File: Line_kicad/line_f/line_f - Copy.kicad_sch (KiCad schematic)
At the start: 15 parts, among them M2 Motor_DC, M3 Motor_DC, SW1 SW_SPST, SW2 SW_SPDT, SW3 SW_Push, SW4 SW_Push, U1 TB6612FNG_LINE, m1 BLACKPILL

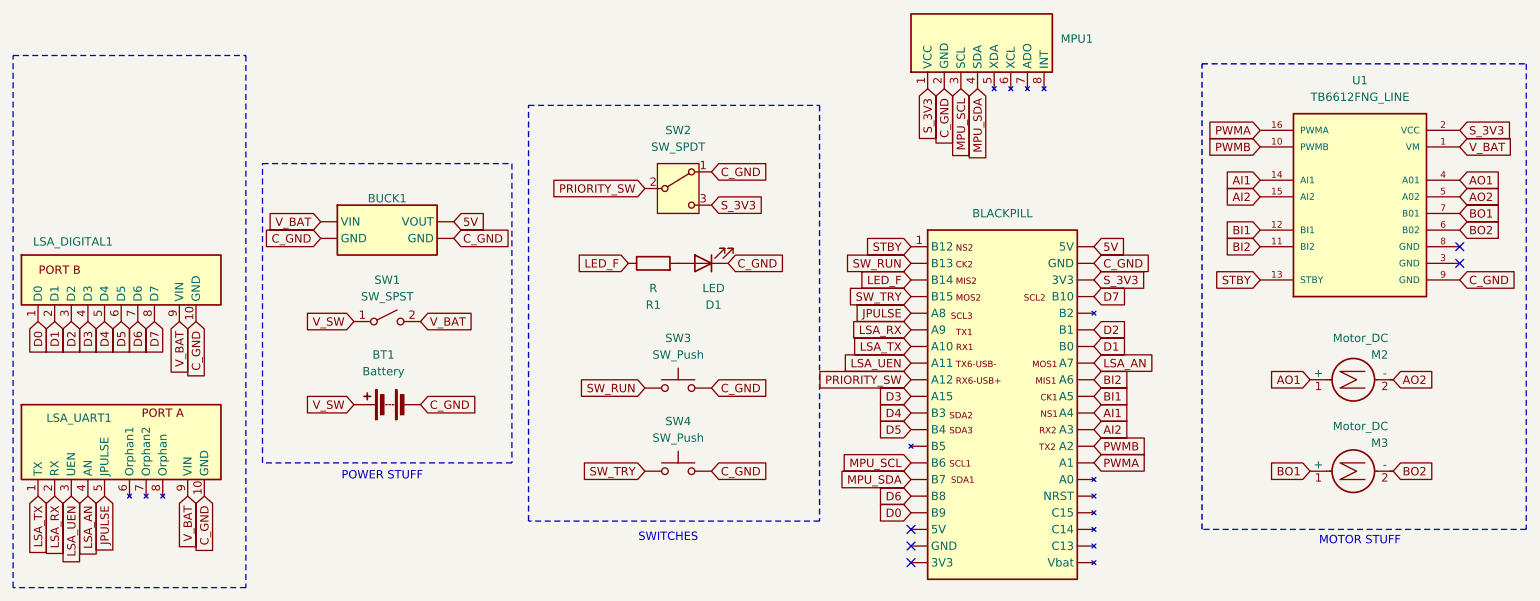
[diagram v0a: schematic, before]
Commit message: 3#
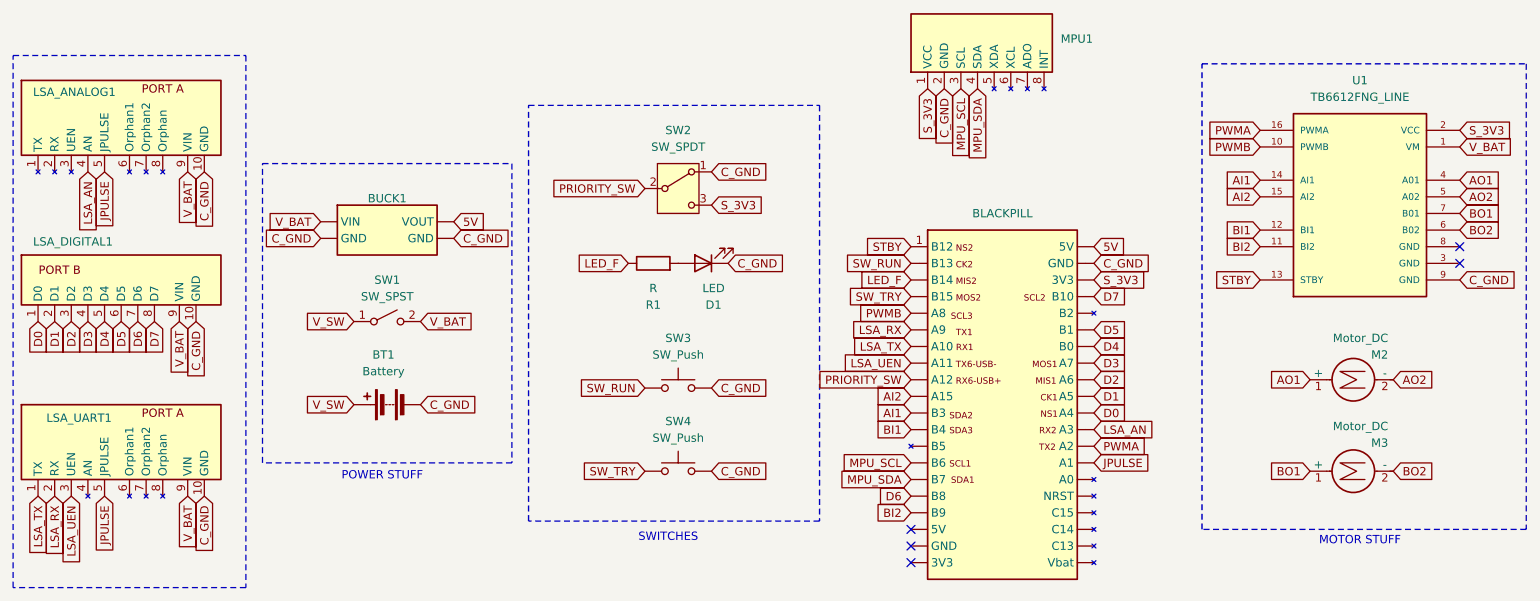
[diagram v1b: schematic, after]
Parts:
- added LSA_ANALOG1: ~, LINE_F_FOOT_LIB:LSA_ANALOG, symbol LINE_F_SYM_LIB:LSA_ANALOG
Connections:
- net AI1: now also m1.11 (B3); no longer m1.31 (A4)
- net AI2: now also m1.10 (A15); no longer m1.32 (A3)
- net BI1: now also m1.12 (B4); no longer m1.30 (A5)
- net BI2: now also m1.17 (B9); no longer m1.29 (A6)
- net C_GND: now also LSA_ANALOG1.10 (GND)
- net D0: now also m1.31 (A4); no longer m1.17 (B9)
- net D1: now also m1.30 (A5); no longer m1.27 (B0)
- net D2: now also m1.29 (A6); no longer m1.26 (B1)
- net D3: now also m1.28 (A7); no longer m1.10 (A15)
- net D4: now also m1.27 (B0); no longer m1.11 (B3)
- net D5: now also m1.26 (B1); no longer m1.12 (B4)
- net JPULSE: now also m1.34 (A1), LSA_ANALOG1.5 (JPULSE); no longer m1.5 (A8)
- net LSA_AN: now also m1.32 (A3), LSA_ANALOG1.4 (AN); no longer LSA_UART1.4 (AN), m1.28 (A7)
- net PWMA: now also m1.33 (A2); no longer m1.34 (A1)
- net PWMB: now also m1.5 (A8); no longer m1.33 (A2)
- net V_BAT: now also LSA_ANALOG1.9 (VIN)
